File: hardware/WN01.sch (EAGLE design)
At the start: 33 parts, among them J1 AUDIO-JACK2PTH, J2 M04X2, Q1 G2XX3---PW20, Q4 32.768 kHz, U1 MIC5025-3.3

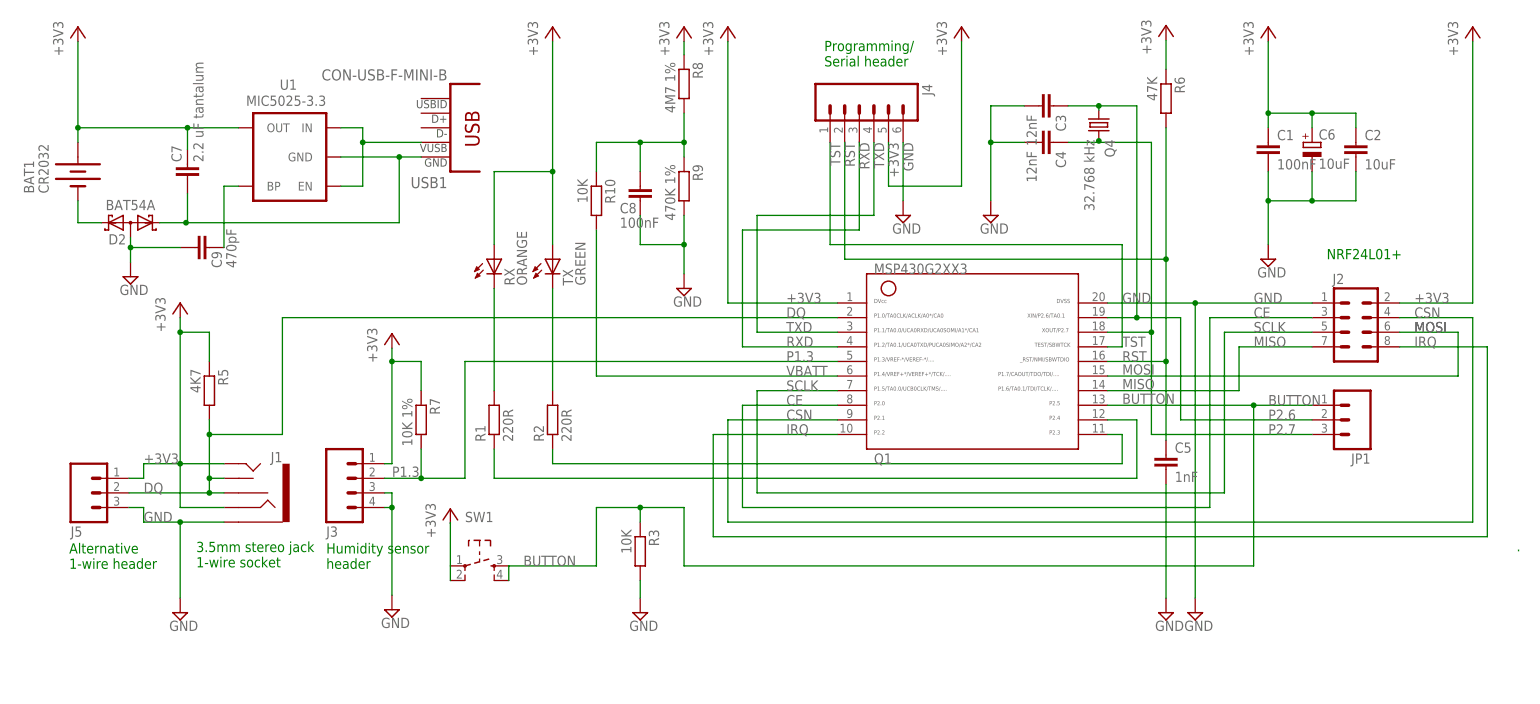
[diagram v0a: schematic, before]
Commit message: version WN01, first draft
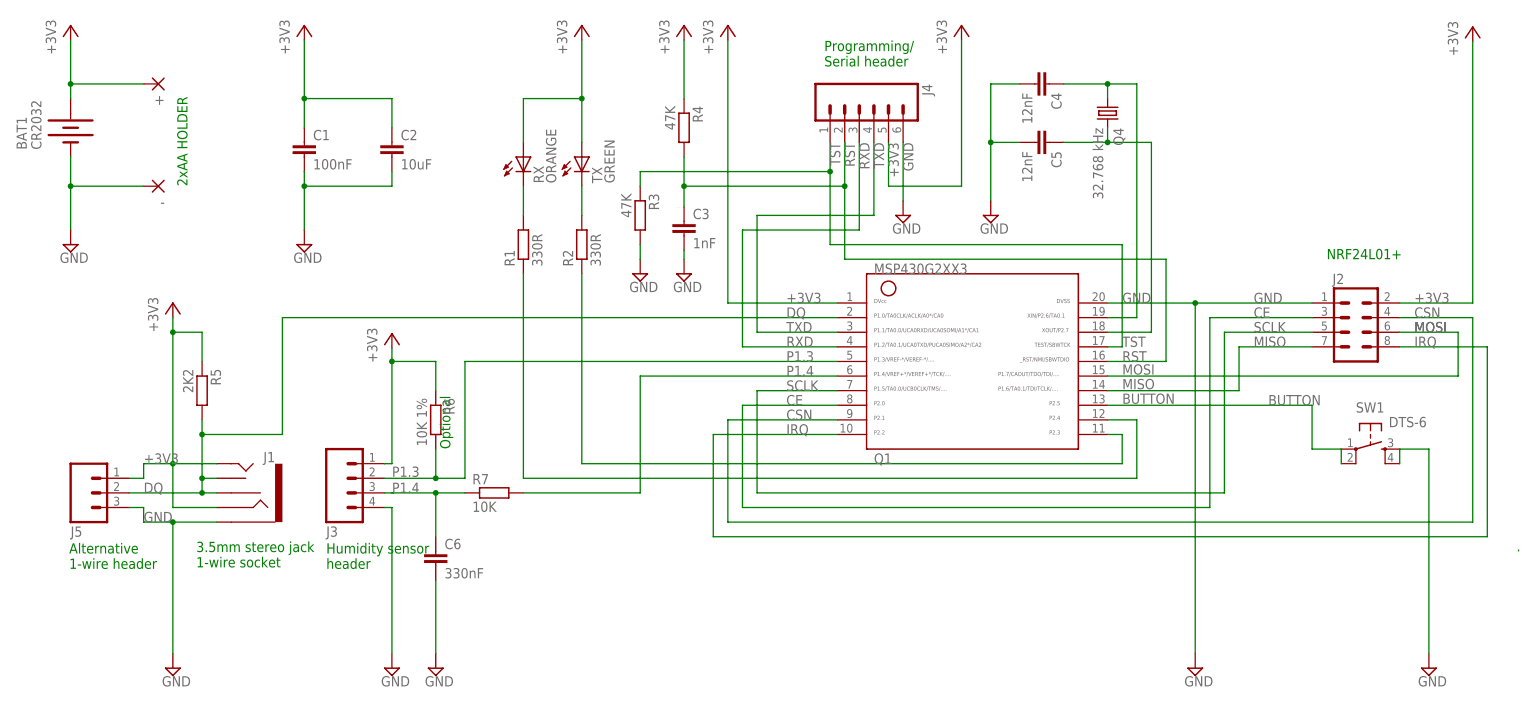
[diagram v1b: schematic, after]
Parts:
- removed C7: 2.2 uF tantalum, rcl:C-EUC1206
- removed C8: 100nF, resistor:C-EUC0805
- removed C9: 470pF, resistor:C-EUC0805
- removed D2: BAT54A, diode:BAT54A
- removed JP1: (no value), SparkFun:M03PTH
- removed R10: 10K, resistor:R-EU_M0805
- removed R8: 4M7 1%, resistor:R-EU_M0805
- removed R9: 470K 1%, resistor:R-EU_M0805
- removed U1: MIC5025-3.3, SparkFun:V_REG_LDOSMD
- removed USB1: CON-USB-F-MINI-B, dp_devices:CON-USB-F-MINI-B
- added +, -: (no value), wirepad:2,54/1,0
- added R4: 47K, resistor:R-EU_M0805
- C3: value 12nF -> 1nF
- C5: value 1nF -> 12nF
- C6: value 10uF -> 330nF; device rcl:CPOL-EUE2.5-7 -> resistor:C-EUC0805
- R1, R2: value 220R -> 330R
- R3: value 10K -> 47K
- R5: value 4K7 -> 2K2
- R6: value 47K -> 10K 1%
- R7: value 10K 1% -> 10K
- SW1: value (none) -> DTS-6; device dp_devices:SW_TACT_4P -> switch-tact:DTS-6
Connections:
- removed net N$11: C7.2, D2.K1, U1.GND, USB1USB.GND
- removed net N$12: U1.EN, U1.IN, USB1USB.VUSB
- removed net N$13: BAT1.-, D2.K2
- removed net N$15: C9.2, U1.BP
- removed net VBATT: Q1.6, R10.2
- removed net VBATT1: C8.1, R10.1, R8.2, R9.1
- new net N$7: C6.1, J3.3, R7.1
- new net P1.4: Q1.6, R7.2
- net +3V3: now also +.P, R4.1; no longer C6.+, C7.1, R7.1, R8.1, SW1.1, SW1.2, U1.OUT
- net BUTTON: now also SW1.1, SW1.2; no longer JP1.1, R3.1, SW1.3, SW1.4
- net GND: now also -.P, BAT1.-, C6.2, SW1.3, SW1.4; no longer C6.-, C8.2, C9.1, D2.AA, J3.3, R9.2
- net P1.3: now also R6.2; no longer R7.2
- net P2.6: now also C4.1; no longer C3.1, JP1.2
- net P2.7: now also C5.1; no longer C4.1, JP1.3
- net RST: now also C3.1, R4.2; no longer C5.1, R6.2
- net TST: now also R3.1
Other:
- note added: "2xAA HOLDER"
- note added: "Optional"
- moved on the sheet: BAT1, C1, C2, C3, C4, C5, J1, Q4, R1, R2, R3, R5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
